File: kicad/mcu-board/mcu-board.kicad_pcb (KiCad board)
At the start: 2 copper layers, 54.5 x 46.3 mm, 65 parts, among them J10 Conn_01x02, J11 Conn_01x02, J12 UJ20-C-H-G-SMT-P16-TR, J13 Conn_01x06, J2 Conn_01x06, J3 Conn_01x01, J4 Conn_01x02, J5 Conn_01x02, J6 Conn_01x02, J7 Conn_01x03, J8 Conn_01x04, J9 Conn_01x02, Q1 Q_NPN_CEB, SW1 SW_Push, SW2 SW_Push, U1 Lora1276-C1-868, U2 ESP32-S3-WROOM-1U-N16R8, U3 LM66200DRLR, U4 AP3445LW6-7

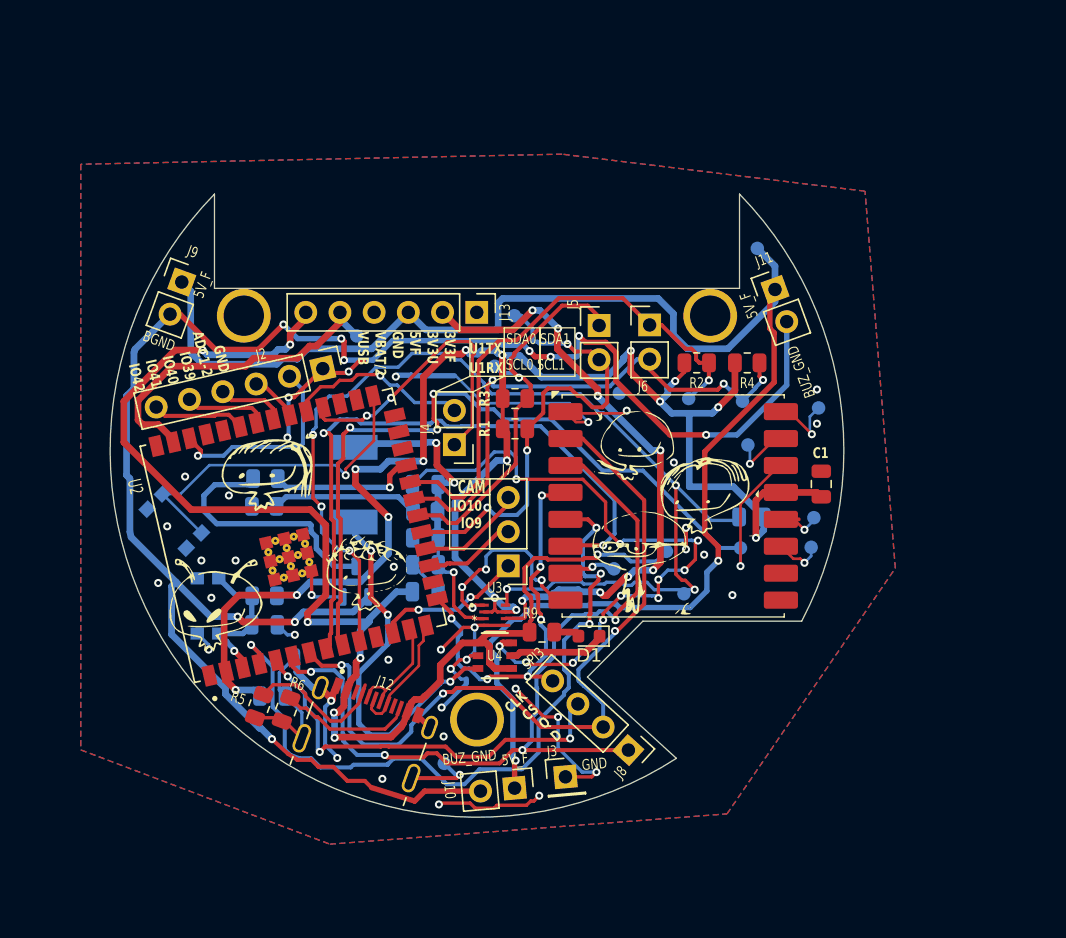
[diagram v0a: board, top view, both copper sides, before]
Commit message: feat: finished pcb, might add more artwork later?
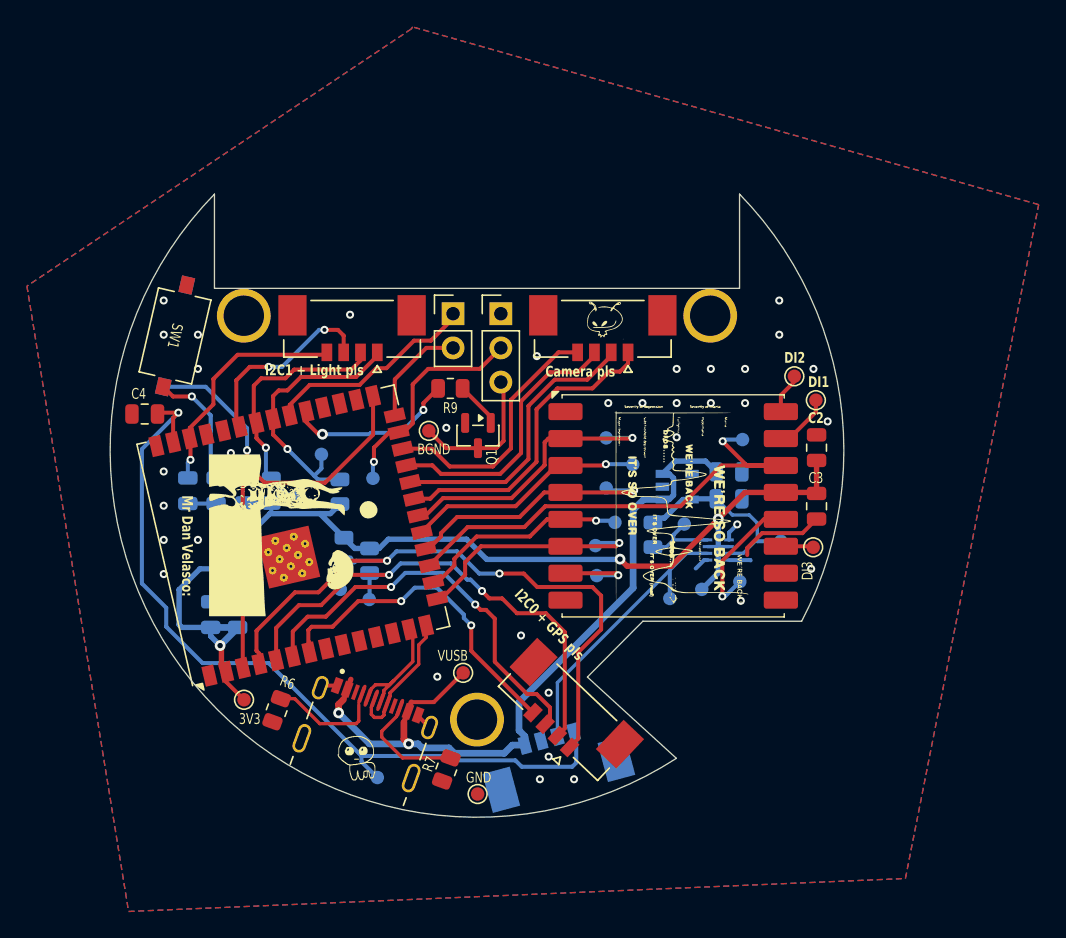
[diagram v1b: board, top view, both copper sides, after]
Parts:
- removed the C6 at (100.8, 109.0)
- removed D1: LED, LED_SMD:LED_0603_1608Metric
- removed the G*** at (83.6, 109.0)
- removed the G*** at (121.7, 101.8)
- removed the G*** at (89.4, 100.2)
- removed the G*** at (116.5, 106.5)
- removed the G*** at (96.7, 107.5)
- removed the G*** at (116.5, 98.2)
- removed J10, J11, J9: Conn_01x02, Connector_PinHeader_2.54mm:PinHeader_1x02_P2.54mm_Vertical
- removed J13: Conn_01x06, Connector_PinHeader_2.54mm:PinHeader_1x06_P2.54mm_Vertical
- removed the J6 at (117.5, 89.2)
- removed J8: Conn_01x04, Connector_PinHeader_2.54mm:PinHeader_1x04_P2.54mm_Vertical
- removed L1: 2u2H, PSAT_Library:IND_SPM6530T-1R5M100
- removed the R7 at (100.8, 103.0)
- removed the R8 at (88.9, 102.7)
- removed the R9 at (109.5, 112.0)
- removed the TP15 at (120.4, 94.7)
- added C7: 0.1uf, Capacitor_SMD:C_0805_2012Metric, B.Cu at (84.9, 110.7)
- added C8: 1u, Capacitor_SMD:C_0805_2012Metric, B.Cu at (123.4, 100.1)
- added C9: 1u, Capacitor_SMD:C_0805_2012Metric, B.Cu at (123.4, 102.1)
- added G***: LOGO, LOGO, F.Cu at (95.8, 121.3)
- added G***: LOGO, LOGO, B.Cu at (112.0, 94.2)
- added G***: LOGO, LOGO, F.Cu at (119.2, 102.5)
- added G***: LOGO, LOGO, F.Cu at (113.5, 88.4)
- added G***: LOGO, LOGO, F.Cu at (91.5, 104.8)
- added G***: LOGO, LOGO, B.Cu at (117.0, 89.5)
- added G***: LOGO, LOGO, B.Cu at (110.4, 90.3)
- added G***: LOGO, LOGO, B.Cu at (117.2, 94.9)
- added G***: LOGO, LOGO, B.Cu at (113.3, 89.5)
- added G***: LOGO, LOGO, B.Cu at (114.3, 92.3)
- added J1: Conn_01x03, Connector_PinHeader_2.54mm:PinHeader_1x03_P2.54mm_Vertical, F.Cu at (106.5, 88.3)
- added TP15: TestPoint, TestPoint:TestPoint_Pad_D1.0mm, B.Cu at (121.4, 108.8)
- added TP15: TestPoint, TestPoint:TestPoint_Pad_D1.0mm, B.Cu at (113.6, 107.8)
- added TP17: TestPoint, TestPoint:TestPoint_Pad_D1.0mm, F.Cu at (103.7, 115.0)
- added TP18: TestPoint, TestPoint:TestPoint_Pad_D1.0mm, F.Cu at (104.7, 124.0)
- added TP19: TestPoint, TestPoint:TestPoint_Pad_D1.0mm, F.Cu at (87.4, 117.0)
- added TP20: TestPoint, TestPoint:TestPoint_Pad_D1.0mm, B.Cu at (120.1, 104.0)
- added TP21: TestPoint, TestPoint:TestPoint_Pad_D1.0mm, B.Cu at (127.2, 105.2)
- added TP22: TestPoint, TestPoint:TestPoint_Pad_D1.0mm, B.Cu at (119.0, 109.5)
- added TP23: TestPoint, TestPoint:TestPoint_Pad_D1.0mm, F.Cu at (101.1, 97.0)
- added VBAT1: TestPoint, TestPoint:TestPoint_Pad_D1.0mm, B.Cu at (97.3, 122.8)
- C1: renamed from C7; value 0.1uf -> 1uf
- C3, C4: value 22uF -> 0.1uf; moved to F.Cu
- C5: value 22pF -> 0.1uf
- J2: value Conn_01x06 -> Conn_01x02; footprint Connector_PinHeader_2.54mm:PinHeader_1x06_P2.54mm_Vertical -> Connector_PinHeader_2.54mm:PinHeader_1x02_P2.54mm_Vertical
- J3: value Conn_01x01 -> 533980471; footprint Connector_PinHeader_2.54mm:PinHeader_1x01_P2.54mm_Vertical -> PSAT_Library:MOLEX_533980471
- J4, J5: value Conn_01x02 -> 533980471; footprint Connector_PinHeader_2.54mm:PinHeader_1x02_P2.54mm_Vertical -> PSAT_Library:MOLEX_533980471
- J7: value Conn_01x03 -> 533980471; footprint Connector_PinHeader_2.54mm:PinHeader_1x03_P2.54mm_Vertical -> PSAT_Library:MOLEX_533980471; moved to B.Cu
- Q1: value Q_NPN_CEB -> MMBT619; footprint Package_TO_SOT_SMD:SOT-23-3 -> Package_TO_SOT_SMD:SOT-23; moved to F.Cu
- R1, R2, R3, R4: value 4.7k -> 5.1k; moved to B.Cu
- R5: renamed from R11; value 5.1k -> 10k
- R9: renamed from R10; moved to F.Cu
- SW1: footprint Button_Switch_SMD:SW_Push_1P1T_NO_CK_KMR2 -> Button_Switch_SMD:SW_Tactile_SPST_NO_Straight_CK_PTS636Sx25SMTRLFS; moved to F.Cu
- SW2: footprint Button_Switch_SMD:SW_Push_1P1T_NO_CK_KMR2 -> Button_Switch_SMD:SW_Tactile_SPST_NO_Straight_CK_PTS636Sx25SMTRLFS
- TP11, TP12, TP13: moved to F.Cu
- U2: footprint PSAT_Library:XCVR_ESP32-S3-WROOM-1U-N16R8 -> footprints2:ESP32-S3-WROOM-1U
- U3: footprint footprints:SOT-5X3_DRL_TEX -> footprints2:SOT-5X3_DRL_TEX; moved to B.Cu
- U4: value AP3445LW6-7 -> TLV75733PDBVR; footprint PSAT_Library:SOT26_AP3445_DIO-L -> footprints2:TLV75733PDBVR; moved to B.Cu
- moved TP5 37.1 mm to (93.1, 98.8)
- moved R2 33.0 mm to (89.4, 101.5), turned to -90 degrees
- moved TP6 33.0 mm to (97.0, 100.6)
- moved TP4 32.1 mm to (94.5, 108.8)
- moved TP13 31.8 mm to (129.7, 105.7), turned to 0 degrees
- moved R4 31.7 mm to (94.5, 101.6), turned to 90 degrees
- moved C3 29.4 mm to (129.9, 102.7), turned to -90 degrees
- moved TP14 24.8 mm to (124.2, 108.2)
- moved TP10 23.7 mm to (114.9, 103.8)
- moved C4 22.8 mm to (80.0, 95.8), turned to 180 degrees
- moved TP3 20.8 mm to (91.4, 101.8)
- moved SW1 20.2 mm to (82.2, 90.0), turned to -103 degrees
- moved TP2 19.7 mm to (96.7, 109.6)
- moved U4 18.5 mm to (119.5, 101.2), turned to 90 degrees
- moved C5 17.6 mm to (83.2, 101.5), turned to 90 degrees
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- renumbered C1 to C2, C2 to C6, J12 to J6, R5 to R6, R6 to R7, R12 to R8
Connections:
- C3 pad 1: GND -> +3V3
- C3 pad 2: +3V3_USB -> GND
- C4 pad 1: GND -> /VBAT_IO1
- C4 pad 2: +3V3_USB -> GND
- C5 pad 1: +3V3_USB -> GND
- C5 pad 2: Net-(U4-FB) -> /LIGHT_2_ADC1CH1_IO2
- J2 pad 1: GND -> /IO39
- J2 pad 2: /ADC1_CH2 -> /IO45
- J3 pad 1: GND -> /I2C0_SCL_IO4
- J4 pad 1: /U1RX -> /I2C1_SCL_IO40
- J4 pad 2: /U1TX -> /I2C1_SDA_IO41
- J5 pad 1: /I2CEXT0_SDA -> /CAM_IO13
- J5 pad 2: /I2CEXT0_SCL -> /CAM_IO14
- J7 pad 1: /SERVO_PWM -> /VBAT_IO1
- J7 pad 2: /CAM_GPIO9 -> +3V3_PSU_LDO
- J7 pad 3: /CAM_GPIO10 -> GND
- Q1 pad 1: BUZ_GND -> Net-(Q1-B)
- Q1 pad 3: Net-(Q1-B) -> BUZ_GND
- R1 pad 1: /I2CEXT0_SDA -> /I2C0_SDA_IO5
- R2 pad 1: /I2CEXT1_SDA -> /I2C1_SDA_IO41
- R3 pad 2: /I2CEXT0_SCL -> /I2C0_SCL_IO4
- R4 pad 2: /I2CEXT1_SCL -> /I2C1_SCL_IO40
- R8 pad 1: +3V3 -> +3V3_LDO_LOCAL
- R8 pad 2: /POWER_ST -> /Power Management/POWER_ST
- R9 pad 1: /BUZZER -> /BUZZER_IO38
- TP1 pad 1: GND -> /~{LORA_EN}_IO3
- TP10 pad 1: /V_BAT/2 -> /LORA_SPI3_CS_IO46
- TP11 pad 1: /POWER_ST -> /DI1
- TP12 pad 1: V_USB -> /DI2
- TP13 pad 1: GND -> /DI3
- TP14 pad 1: +5V_FUSED -> /DI4
- TP16 pad 1: /I2CEXT1_SCL -> /LORA_IRQ_IO9
- TP2 pad 1: /I2CEXT0_SDA -> /I2C0_SDA_IO5
- TP3 pad 1: /I2CEXT0_SCL -> /I2C1_SDA_IO41
- TP4 pad 1: /DI1 -> /I2C0_SCL_IO4
- TP5 pad 1: /DI2 -> /I2C1_SCL_IO40
- TP6 pad 1: /DI3 -> /SERVO_IO48
- TP7 pad 1: /DI4 -> /LORA_SPI3_Q_IO12
- TP8 pad 1: /LoRa_IRQ -> /LORA_SPI3_D_IO11
- TP9 pad 1: /DI5 -> /LORA_SPI3_CLK_IO10
- U1 pad 14: /LoRa_IRQ -> /LORA_IRQ_IO9
- U1 pad 2: /SPI3_Q -> /LORA_SPI3_Q_IO12
- U1 pad 3: /SPI3_D -> /LORA_SPI3_D_IO11
- U1 pad 4: /SPI3_CLK -> /LORA_SPI3_CLK_IO10
- U1 pad 5: /SPI3_CS0_O -> /LORA_SPI3_CS_IO46
- U1 pad 6: /~{LoRa_EN} -> /~{LORA_EN}_IO3
- U2 pad 10: /POWER_ST -> unconnected-(U2-IO17-Pad10)
- U2 pad 12: /SERVO_PWM -> unconnected-(U2-IO8-Pad12)
- U2 pad 15: /SPI3_CLK -> /~{LORA_EN}_IO3
- U2 pad 16: unconnected-(U2-IO46-Pad16) -> /LORA_SPI3_CS_IO46
- U2 pad 17: /CAM_GPIO9 -> /LORA_IRQ_IO9
- U2 pad 18: /CAM_GPIO10 -> /LORA_SPI3_CLK_IO10
- U2 pad 19: /I2CEXT0_SCL -> /LORA_SPI3_D_IO11
- U2 pad 20: /I2CEXT0_SDA -> /LORA_SPI3_Q_IO12
- U2 pad 21: /I2CEXT1_SCL -> /CAM_IO13
- U2 pad 22: /I2CEXT1_SDA -> /CAM_IO14
- U2 pad 23: /BUZZER -> /CAM_IO21
- U2 pad 24: unconnected-(U2-IO47-Pad24) -> /CAM_IO47
- U2 pad 25: unconnected-(U2-IO48-Pad25) -> /SERVO_IO48
- U2 pad 26: unconnected-(U2-IO45-Pad26) -> /IO45
- U2 pad 30: /U1RX -> unconnected-(U2-IO37-Pad30)
- U2 pad 31: /U1TX -> /BUZZER_IO38
- U2 pad 32: /GPIO39 -> /IO39
- U2 pad 33: /GPIO40 -> /I2C1_SCL_IO40
- U2 pad 34: /GPIO41 -> /I2C1_SDA_IO41
- U2 pad 35: /GPIO42 -> /LIGHT_1_IO42
- U2 pad 38: /ADC1_CH2 -> /LIGHT_2_ADC1CH1_IO2
- U2 pad 39: /V_BAT/2 -> /VBAT_IO1
- U2 pad 4: /SPI3_CS0_O -> /I2C0_SCL_IO4
- U2 pad 5: /SPI3_CS1_O -> /I2C0_SDA_IO5
- U2 pad 6: /SPI3_D -> /GPS_U1TX_IO6
- U2 pad 7: /SPI3_Q -> /GPS_U1RX_IO7
- U2 pad 8: /~{LoRa_EN} -> unconnected-(U2-IO15-Pad8)
- U2 pad 9: /LoRa_IRQ -> unconnected-(U2-IO16-Pad9)
- U3 pad 3: +3V3_USB -> +3V3_LDO_LOCAL
- U3 pad 6: +3V3_PSU_UNFUSED -> +3V3_PSU_LDO
- U3 pad 8: /POWER_ST -> /Power Management/POWER_ST
- U4 pad 3: Net-(U4-LX) -> V_USB
- U4 pad 4: V_USB -> unconnected-(U4-NC-Pad4)
- U4 pad 5: Net-(D1-K) -> +3V3_LDO_LOCAL
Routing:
- net BUZ_GND: track 128.3 -> 10.8 mm, vias 10 -> 0
- net +5V_FUSED: track 117.1 -> 0.00 mm, vias 2 -> 0
- net GND: track 122.7 -> 15.4 mm, vias 44 -> 35
- net /POWER_ST: track 82.1 -> 0.00 mm, vias 6 -> 0
- net /LoRa_IRQ: track 63.9 -> 0.00 mm, vias 4 -> 0
- net Net-(U4-FB): track 62.7 -> 0.00 mm, vias 11 -> 0
- net /SPI3_D: track 62.5 -> 0.00 mm, vias 4 -> 0
- net /VBAT_IO1: track 0.00 -> 61.0 mm, vias 0 -> 1
- net /SPI3_Q: track 58.2 -> 0.00 mm, vias 3 -> 0
- net /SPI3_CS0_O: track 55.7 -> 0.00 mm, vias 4 -> 0
- net /I2C0_SCL_IO4: track 0.00 -> 49.6 mm, vias 0 -> 2
- net /~{LoRa_EN}: track 48.0 -> 0.00 mm, vias 2 -> 0
- net V_USB: track 100.9 -> 54.6 mm, vias 7 -> 2
- net +3V3_PSU_UNFUSED: track 45.8 -> 0.00 mm, vias 8 -> 0
- net +3V3: track 130.0 -> 84.3 mm, vias 15 -> 3
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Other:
- board text added: "3V3"
- board text added: "3V3_LDO"
- board text added: "3V3_PSU"
- board text added: "CS"
- board text added: "Camera pls"
- board text added: "DI3"
- board text added: "DI4"
- board text added: "Daniel still gotta eat the 2x buldak"
- board text added: "Dedicated to: mr long schlong"
- board text added: "I2C0 + GPS pls"
- board text added: "I2C0_SCL"
- board text added: "I2C0_SDA"
- board text added: "I2C1 + Light pls"
- board text added: "I2C1_SCL"
- board text added: "I2C1_SDA"
- board text added: "IO48"
- board text added: "MCU-BOARD REV 2"
- board text added: "Mr Dan Velasco:"
- board text added: "PST"
- board text added: "Power here pls"
- board text added: "RX_IRQ"
- board text added: "SCLK"
- board text added: "SPID"
- board text added: "SPIQ"
- board text added: "VBAT"
- board text added: "VUSB"
- board text added: "desinged by aids"
- board text added: "~{EN}"
- board text removed: "3V3F 3V3U 5VF GND VBAT/2 VUSB"
- board text removed: "5VF"
- board text removed: "5V_F"
- board text removed: "BOOT"
- board text removed: "BUZ_GND"
- board text removed: "CAM"
- board text removed: "CLK CS Q D"
- board text removed: "DI4 DI3"
- board text removed: "Designed by: aids (might be cooked)"
- board text removed: "EN"
- board text removed: "GND ADC1-2 IO39 IO40 IO41 IO42"
- board text removed: "IO10 IO9"
- board text removed: "LoRa_IRQ"
- board text removed: "MCU-BOARD REV 1"
- board text removed: "POWER_ST"
- board text removed: "SCL0"
- board text removed: "SCL0 SCL1"
- board text removed: "SCL1"
- board text removed: "SDA0"
- board text removed: "SDA0 SDA1"
- board text removed: "SDA1"
- board text removed: "SPI3"
- board text removed: "U1RX"
- board text removed: "U1TX"
- board text removed: "VBAT/2"
- board text removed: "V_USB"
- board text removed: "{dblquote}I apologise Miguel{dblquote}"
